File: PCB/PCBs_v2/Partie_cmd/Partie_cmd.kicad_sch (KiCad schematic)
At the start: 74 parts, among them J1 Barrel_Jack, J10 Conn_01x02, J2 Conn_01x04_Socket, J3 Conn_01x04_Socket, J4 Conn_01x12, J6 Conn_01x04, J7 Conn_01x04, J9 Conn_01x02, U1 ESP32-S3-DEVKITC-1-N8R2, U2 BU18SD5WG-TL, U3 BU33SD5WG-TR, U4 XL1509-5.0

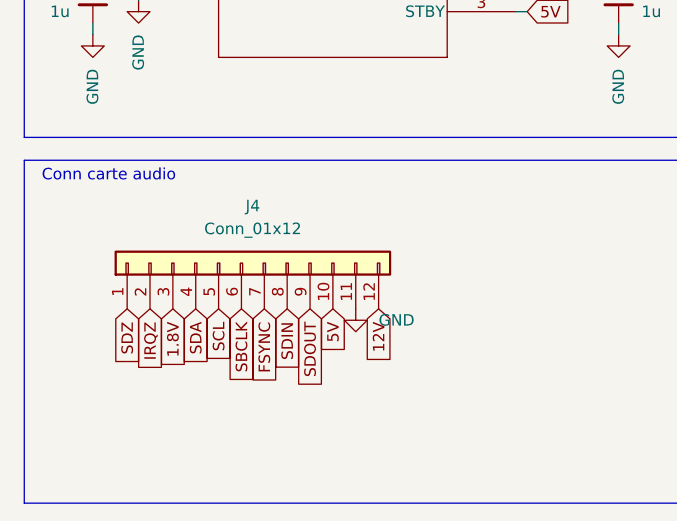
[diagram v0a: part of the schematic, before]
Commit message: fin du routage
svpsvpsvpsvpsvp
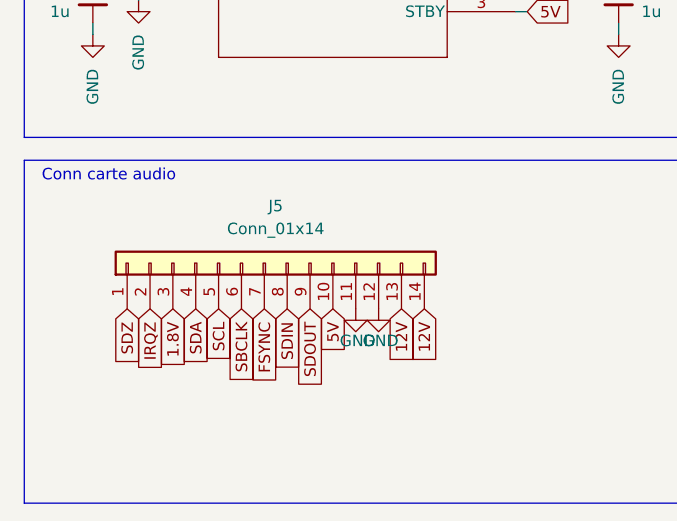
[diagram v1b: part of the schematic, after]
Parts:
- removed J4: Conn_01x12, Connector_PinHeader_1.27mm:PinHeader_1x12_P1.27mm_Vertical, symbol Connector_Generic:Conn_01x12
- added J5: Conn_01x14, Connector_PinHeader_1.27mm:PinHeader_1x14_P1.27mm_Vertical, symbol Connector_Generic:Conn_01x14
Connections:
- net 1.8V: now also J5.3 (Pin_3)
- net 12V: now also J5.13 (Pin_13), J5.14 (Pin_14)
- net 5V: now also J5.10 (Pin_10)
- net FSYNC: now also J5.7 (Pin_7)
- net GND: now also J5.11 (Pin_11), J5.12 (Pin_12)
- net IRQZ: now also J5.2 (Pin_2)
- net SBCLK: now also J5.6 (Pin_6)
- net SCL: now also J5.5 (Pin_5)
- net SDA: now also J5.4 (Pin_4)
- net SDIN: now also J5.8 (Pin_8)
- net SDOUT: now also J5.9 (Pin_9)
- net SDZ: now also J5.1 (Pin_1)
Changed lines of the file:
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@@
 		)
 	)
+	(global_label "12V"
+		(shape input)
+		(at 63.5 166.37 270)
+		(fields_autoplaced yes)
+		(effects
+			(font
+				(size 1.27 1.27)
+			)
+			(justify right)
+		)
+		(property "Intersheetrefs" "${INTERSHEET_REFS}"
+			(at 63.5 172.8628 90)
+			(effects
+				(font
+					(size 1.27 1.27)
+				)
+				(justify right)
+				(hide yes)
+			)
+		)
+	)
 	(global_label "SDZ"
 		(shape input)
@@
 	(global_label "12V"
 		(shape input)
-		(at 58.42 166.37 270)
+		(at 60.96 166.37 270)
 		(fields_autoplaced yes)
 		(effects
@@
 		)
 		(property "Intersheetrefs" "${INTERSHEET_REFS}"
-			(at 58.42 172.8628 90)
+			(at 60.96 172.8628 90)
 			(effects
 				(font
@@
 	)
 	(symbol
+		(lib_id "Connector_Generic:Conn_01x14")
+		(at 45.72 161.29 90)
+		(unit 1)
+		(exclude_from_sim no)
+		(in_bom yes)
+		(on_board yes)
+		(dnp no)
+		(fields_autoplaced yes)
+		(property "Reference" "J5"
+			(at 46.99 154.94 90)
+			(effects
+				(font
+					(size 1.27 1.27)
+				)
+			)
+		)
+		(property "Value" "Conn_01x14"
+			(at 46.99 157.48 90)
+			(effects
+				(font
+					(size 1.27 1.27)
+				)
+			)
+		)
+		(property "Footprint" "Connector_PinHeader_1.27mm:PinHeader_1x14_P1.27mm_Vertical"
+			(at 45.72 161.29 0)
+			(effects
+				(font
+					(size 1.27 1.27)
+				)
+				(hide yes)
+			)
+		)
+		(property "Datasheet" "~"
+			(at 45.72 161.29 0)
+			(effects
+				(font
+					(size 1.27 1.27)
+				)
+				(hide yes)
+			)
+		)
+		(property "Description" "Generic connector, single row, 01x14, script generated (kicad-library-utils/schlib/autogen/connector/)"
+			(at 45.72 161.29 0)
+			(effects
+				(font
+					(size 1.27 1.27)
+				)
+				(hide yes)
+			)
+		)
+		(pin "4"
+		)
+		(pin "2"
+		)
+		(pin "7"
+		)
+		(pin "1"
+		)
+		(pin "3"
+		)
+		(pin "5"
+		)
+		(pin "6"
+		)
+		(pin "8"
+		)
+		(pin "9"
+		)
+		(pin "10"
+		)
+		(pin "11"
+		)
+		(pin "14"
+		)
+		(pin "13"
+		)
+		(pin "12"
+		)
+		(instances
+			(project ""
+				(path "/feb16e15-81d7-49b9-8315-2aeb60da597a"
+					(reference "J5")
+					(unit 1)
+				)
+			)
+		)
+	)
+	(symbol
 		(lib_id "Device:LED_Small")
 		(at 208.28 127 270)
@@
 		(on_board yes)
 		(dnp no)
-		(fields_autoplaced yes)
 		(property "Reference" "#PWR022"
 			(at 55.88 172.72 0)
@@
 		)
 		(property "Value" "GND"
-			(at 58.42 167.6399 0)
+			(at 54.102 169.926 0)
 			(effects
 				(font
@@
 	)
 	(symbol
+		(lib_id "power:GND")
+		(at 58.42 166.37 0)
+		(unit 1)
+		(exclude_from_sim no)
+		(in_bom yes)
+		(on_board yes)
+		(dnp no)
+		(property "Reference" "#PWR024"
+			(at 58.42 172.72 0)
+			(effects
+				(font
+					(size 1.27 1.27)
+				)
+				(hide yes)
+			)
+		)
+		(property "Value" "GND"
+			(at 56.642 169.926 0)
+			(effects
+				(font
+					(size 1.27 1.27)
+				)
+				(justify left)
+			)
+		)
+		(property "Footprint" ""
+			(at 58.42 166.37 0)
+			(effects
+				(font
+					(size 1.27 1.27)
+				)
+				(hide yes)
+			)
+		)
+		(property "Datasheet" ""
+			(at 58.42 166.37 0)
+			(effects
+				(font
+					(size 1.27 1.27)
+				)
+				(hide yes)
+			)
+		)
+		(property "Description" "Power symbol creates a global label with name \"GND\" , ground"
+			(at 58.42 166.37 0)
+			(effects
+				(font
+					(size 1.27 1.27)
+				)
+				(hide yes)
+			)
+		)
+		(pin "1"
+		)
+		(instances
+			(project "Partie_cmd"
+				(path "/feb16e15-81d7-49b9-8315-2aeb60da597a"
+					(reference "#PWR024")
+					(unit 1)
+				)
+			)
+		)
+	)
+	(symbol
 		(lib_id "Jumper:SolderJumper_2_Open")
 		(at 142.24 43.18 0)
@@
 					(unit 1)
 				)
-			)
-		)
-	)
-	(symbol
-		(lib_id "Connector_Generic:Conn_01x12")
-		(at 43.18 161.29 90)
-		(unit 1)
-		(exclude_from_sim no)
-		(in_bom yes)
-		(on_board yes)
-		(dnp no)
-		(fields_autoplaced yes)
-		(property "Reference" "J4"
-			(at 44.45 154.94 90)
-			(effects
-				(font
-					(size 1.27 1.27)
-				)
-			)
-		)
-		(property "Value" "Conn_01x12"
-			(at 44.45 157.48 90)
-			(effects
-				(font
-					(size 1.27 1.27)
-				)
-			)
-		)
-		(property "Footprint" "Connector_PinHeader_1.27mm:PinHeader_1x12_P1.27mm_Vertical"
-			(at 43.18 161.29 0)
-			(effects
-				(font
-					(size 1.27 1.27)
-				)
-				(hide yes)
-			)
-		)
-		(property "Datasheet" "~"
-			(at 43.18 161.29 0)
-			(effects
-				(font
-					(size 1.27 1.27)
-				)
-				(hide yes)
-			)
-		)
-		(property "Description" "Generic connector, single row, 01x12, script generated (kicad-library-utils/schlib/autogen/connector/)"
-			(at 43.18 161.29 0)
-			(effects
-				(font
-					(size 1.27 1.27)
-				)
-				(hide yes)
-			)
-		)
-		(pin "1"
-		)
-		(pin "5"
-		)
-		(pin "2"
-		)
-		(pin "3"
-		)
-		(pin "4"
-		)
-		(pin "6"
-		)
-		(pin "8"
-		)
-		(pin "7"
-		)
-		(pin "9"
-		)
-		(pin "10"
-		)
-		(pin "11"
-		)
-		(pin "12"
-		)
-		(instances
-			(project ""
-				(path "/feb16e15-81d7-49b9-8315-2aeb60da597a"
-					(reference "J4")
-					(unit 1)
-				)
